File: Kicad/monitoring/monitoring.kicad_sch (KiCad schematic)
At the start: 22 parts, among them J1 Module1, J2 Module2, J3 Module3, J4 buttons, J5 Display, J6 Display, J7 DC_in_outout, U1 4052, U3 L7805, U4 L7805

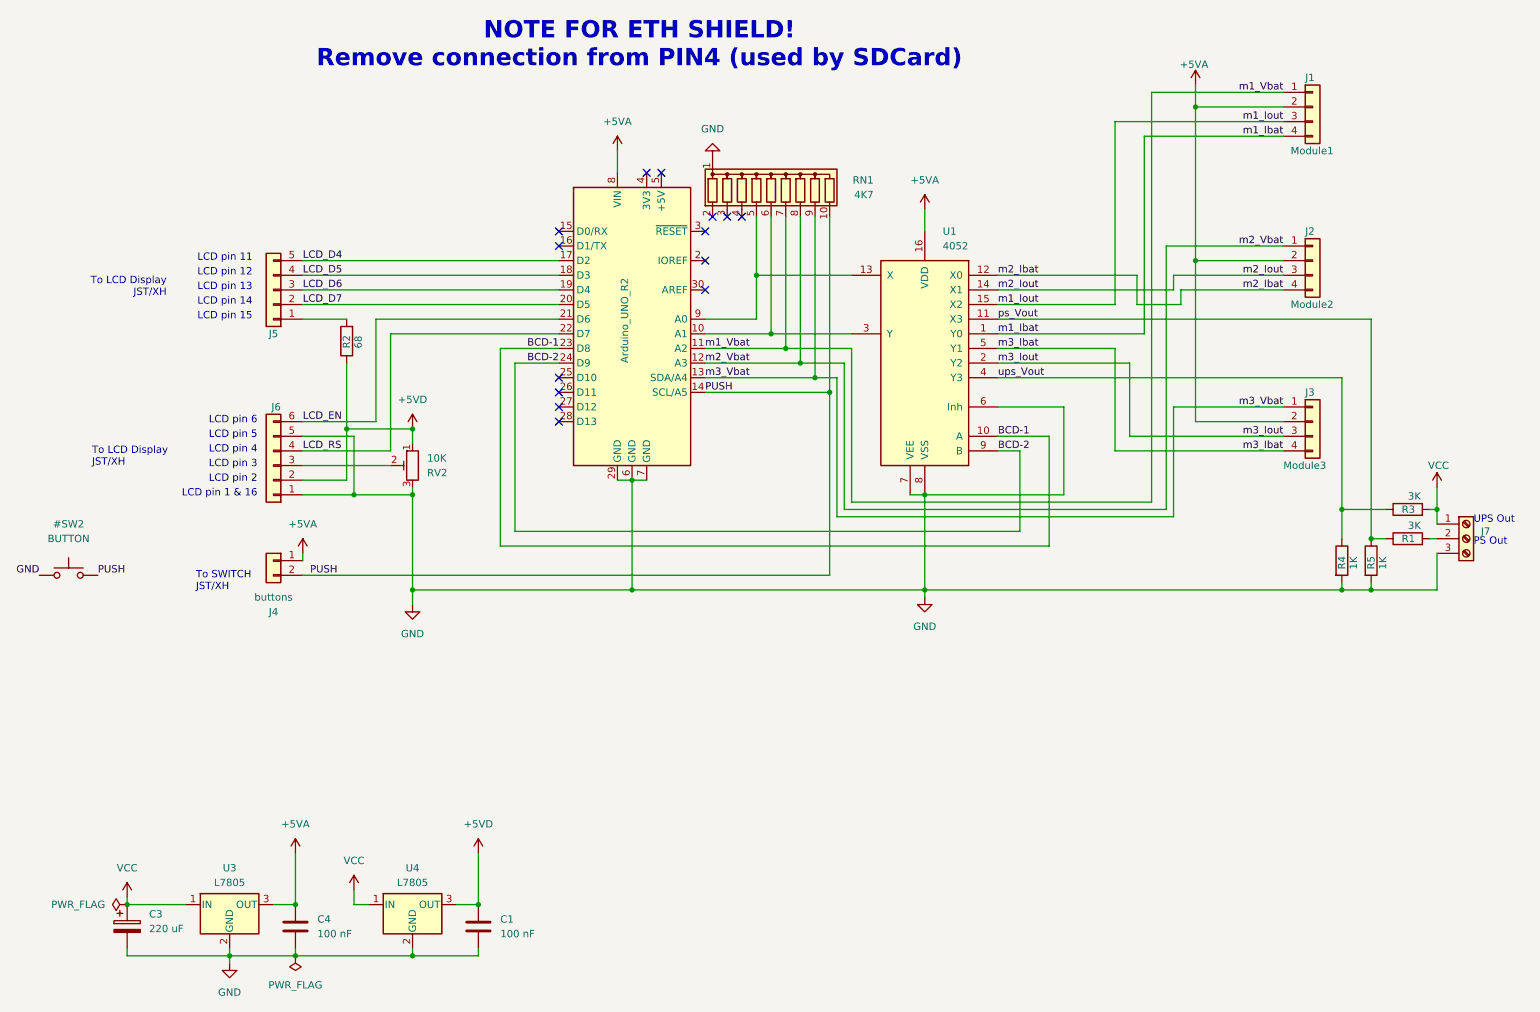
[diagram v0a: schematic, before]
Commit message: Update .sproject, io.cpp, io.h, and 29 more files
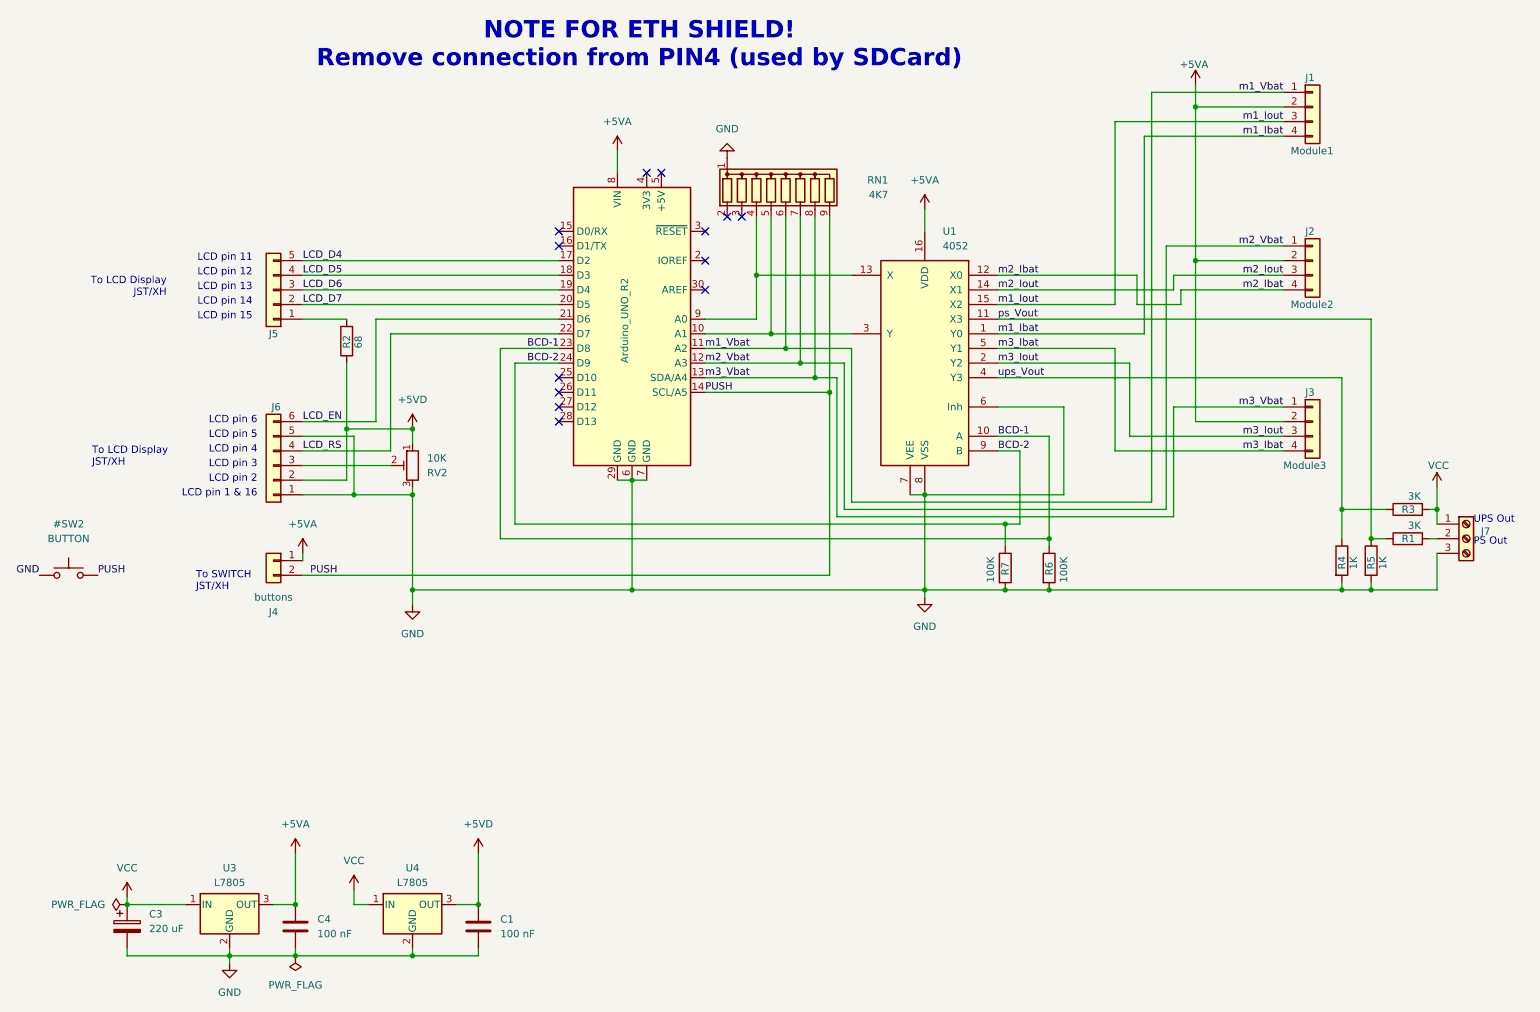
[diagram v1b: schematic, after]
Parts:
- added R6, R7: 100K, Resistor_THT:R_Axial_DIN0204_L3.6mm_D1.6mm_P7.62mm_Horizontal, symbol Device:R
- RN1: footprint Resistor_THT:R_Array_SIP10 -> Resistor_THT:R_Array_SIP8; symbol Device:R_Network09 -> Device:R_Network08
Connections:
- net BCD-1: now also R6.1
- net BCD-2: now also R7.1
- net GND: now also R6.2, R7.2
- net PUSH: now also RN1.9 (R8); no longer RN1.10 (R9)
- net m1_Vbat: now also RN1.6 (R5); no longer RN1.7 (R6)
- net m2_Vbat: now also RN1.7 (R6); no longer RN1.8 (R7)
- net m3_Vbat: now also RN1.8 (R7); no longer RN1.9 (R8)
- net at A1.10 (A1), U1.3 (Y): now also RN1.5 (R4); no longer RN1.6 (R5)
- net at A1.9 (A0), U1.13 (X): now also RN1.4 (R3); no longer RN1.5 (R4)
- no-connect marks 14 -> 13
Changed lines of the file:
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@@
 	)
 	(junction
+		(at 195.58 116.84)
+		(diameter 0)
+		(color 0 0 0 0)
+	)
+	(junction
 		(at 43.18 171.45)
 		(diameter 0)
@@
 	)
 	(junction
+		(at 203.2 116.84)
+		(diameter 0)
+		(color 0 0 0 0)
+	)
+	(junction
+		(at 195.58 105.41)
+		(diameter 0)
+		(color 0 0 0 0)
+	)
+	(junction
 		(at 60.96 180.34)
 		(diameter 0)
@@
 	)
 	(junction
+		(at 203.2 107.95)
+		(diameter 0)
+		(color 0 0 0 0)
+	)
+	(junction
 		(at 130.81 116.84)
 		(diameter 0)
@@
 	)
 	(no_connect
-		(at 144.78 52.07)
-	)
-	(no_connect
 		(at 118.11 87.63)
 	)
@@
 	(wire
 		(pts
-			(xy 110.49 106.68) (xy 198.12 106.68)
-		)
-		(stroke
-			(width 0)
-			(type default)
-		)
-	)
-	(wire
-		(pts
 			(xy 166.37 104.14) (xy 224.79 104.14)
 		)
@@
 	(wire
 		(pts
-			(xy 198.12 92.71) (xy 198.12 106.68)
+			(xy 198.12 92.71) (xy 198.12 105.41)
 		)
 		(stroke
@@
 	(wire
 		(pts
+			(xy 195.58 116.84) (xy 203.2 116.84)
+		)
+		(stroke
+			(width 0)
+			(type default)
+		)
+	)
+	(wire
+		(pts
 			(xy 269.24 107.95) (xy 270.51 107.95)
 		)
@@
 	(wire
 		(pts
+			(xy 195.58 105.41) (xy 198.12 105.41)
+		)
+		(stroke
+			(width 0)
+			(type default)
+		)
+	)
+	(wire
+		(pts
 			(xy 43.18 170.18) (xy 43.18 171.45)
 		)
@@
 	(wire
 		(pts
-			(xy 203.2 109.22) (xy 203.2 90.17)
+			(xy 203.2 109.22) (xy 203.2 107.95)
 		)
 		(stroke
@@
 	(wire
 		(pts
+			(xy 203.2 107.95) (xy 203.2 90.17)
+		)
+		(stroke
+			(width 0)
+			(type default)
+		)
+	)
+	(wire
+		(pts
 			(xy 194.31 92.71) (xy 198.12 92.71)
 		)
@@
 	(wire
 		(pts
+			(xy 110.49 105.41) (xy 195.58 105.41)
+		)
+		(stroke
+			(width 0)
+			(type default)
+		)
+	)
+	(wire
+		(pts
 			(xy 167.64 102.87) (xy 223.52 102.87)
 		)
@@
 	(wire
 		(pts
-			(xy 107.95 109.22) (xy 203.2 109.22)
-		)
-		(stroke
-			(width 0)
-			(type default)
-		)
-	)
-	(wire
-		(pts
 			(xy 220.98 30.48) (xy 243.84 30.48)
 		)
@@
 	(wire
 		(pts
-			(xy 181.61 116.84) (xy 254 116.84)
+			(xy 181.61 116.84) (xy 195.58 116.84)
 		)
 		(stroke
@@
 	(wire
 		(pts
+			(xy 203.2 116.84) (xy 254 116.84)
+		)
+		(stroke
+			(width 0)
+			(type default)
+		)
+	)
+	(wire
+		(pts
 			(xy 226.06 64.77) (xy 243.84 64.77)
 		)
@@
 	(wire
 		(pts
-			(xy 110.49 106.68) (xy 110.49 77.47)
+			(xy 194.31 69.85) (xy 259.08 69.85)
 		)
 		(stroke
@@
 	(wire
 		(pts
-			(xy 194.31 69.85) (xy 259.08 69.85)
+			(xy 214.63 92.71) (xy 243.84 92.71)
 		)
 		(stroke
@@
 	(wire
 		(pts
-			(xy 214.63 92.71) (xy 243.84 92.71)
+			(xy 270.51 102.87) (xy 270.51 105.41)
 		)
 		(stroke
@@
 	(wire
 		(pts
-			(xy 270.51 102.87) (xy 270.51 105.41)
+			(xy 130.81 97.79) (xy 130.81 116.84)
 		)
 		(stroke
@@
 	(wire
 		(pts
-			(xy 130.81 97.79) (xy 130.81 116.84)
+			(xy 72.39 162.56) (xy 72.39 171.45)
 		)
 		(stroke
@@
 	(wire
 		(pts
-			(xy 72.39 162.56) (xy 72.39 171.45)
+			(xy 168.91 101.6) (xy 220.98 101.6)
 		)
 		(stroke
@@
 	(wire
 		(pts
-			(xy 168.91 101.6) (xy 220.98 101.6)
+			(xy 152.4 52.07) (xy 152.4 62.23)
 		)
 		(stroke
@@
 	(wire
 		(pts
-			(xy 152.4 52.07) (xy 152.4 62.23)
+			(xy 195.58 105.41) (xy 195.58 109.22)
 		)
 		(stroke
@@
 	(wire
 		(pts
+			(xy 107.95 107.95) (xy 203.2 107.95)
+		)
+		(stroke
+			(width 0)
+			(type default)
+		)
+	)
+	(wire
+		(pts
+			(xy 110.49 105.41) (xy 110.49 77.47)
+		)
+		(stroke
+			(width 0)
+			(type default)
+		)
+	)
+	(wire
+		(pts
 			(xy 118.11 74.93) (xy 107.95 74.93)
 		)
@@
 	(wire
 		(pts
-			(xy 107.95 74.93) (xy 107.95 109.22)
+			(xy 107.95 74.93) (xy 107.95 107.95)
 		)
 		(stroke
@@
 	)
 	(symbol
+		(lib_id "Device:R")
+		(at 195.58 113.03 0)
+		(unit 1)
+		(exclude_from_sim no)
+		(in_bom yes)
+		(on_board yes)
+		(dnp no)
+		(property "Reference" "R7"
+			(at 195.58 114.3 90)
+			(effects
+				(font
+					(size 1.27 1.27)
+				)
+				(justify left)
+			)
+		)
+		(property "Value" "100K"
+			(at 193.04 115.57 90)
+			(effects
+				(font
+					(size 1.27 1.27)
+				)
+				(justify left)
+			)
+		)
+		(property "Footprint" "Resistor_THT:R_Axial_DIN0204_L3.6mm_D1.6mm_P7.62mm_Horizontal"
+			(at 193.802 113.03 90)
+			(effects
+				(font
+					(size 1.27 1.27)
+				)
+				(hide yes)
+			)
+		)
+		(property "Datasheet" "~"
+			(at 195.58 113.03 0)
+			(effects
+				(font
+					(size 1.27 1.27)
+				)
+				(hide yes)
+			)
+		)
+		(property "Description" "Resistor"
+			(at 195.58 113.03 0)
+			(effects
+				(font
+					(size 1.27 1.27)
+				)
+				(hide yes)
+			)
+		)
+		(pin "2"
+		)
+		(pin "1"
+		)
+		(instances
+			(project "monitoring"
+				(path "/3131f2da-09b7-4506-8682-a60f068b99cd"
+					(reference "R7")
+					(unit 1)
+				)
+			)
+		)
+	)
+	(symbol
 		(lib_id "power:PWR_FLAG")
 		(at 72.39 180.34 180)
@@
 	(symbol
 		(lib_id "power:GND")
-		(at 144.78 41.91 180)
+		(at 147.32 41.91 180)
 		(unit 1)
 		(exclude_from_sim no)
@@
 		(fields_autoplaced yes)
 		(property "Reference" "#PWR09"
-			(at 144.78 35.56 0)
+			(at 147.32 35.56 0)
 			(effects
 				(font
@@
 		)
 		(property "Value" "GND"
-			(at 144.78 36.83 0)
+			(at 147.32 36.83 0)
 			(effects
 				(font
@@
 		)
 		(property "Footprint" ""
-			(at 144.78 41.91 0)
+			(at 147.32 41.91 0)
 			(effects
 				(font
@@
 		)
 		(property "Datasheet" ""
-			(at 144.78 41.91 0)
+			(at 147.32 41.91 0)
 			(effects
 				(font
@@
 		)
 		(property "Description" "Power symbol creates a global label with name \"GND\" , ground"
-			(at 144.78 41.91 0)
+			(at 147.32 41.91 0)
 			(effects
 				(font
@@
 	)
 	(symbol
-		(lib_id "Device:R_Network09")
-		(at 154.94 46.99 0)
+		(lib_id "Device:R")
+		(at 203.2 113.03 0)
+		(unit 1)
+		(exclude_from_sim no)
+		(in_bom yes)
+		(on_board yes)
+		(dnp no)
+		(property "Reference" "R6"
+			(at 203.2 114.3 90)
+			(effects
+				(font
+					(size 1.27 1.27)
+				)
+				(justify left)
+			)
+		)
+		(property "Value" "100K"
+			(at 205.74 115.57 90)
+			(effects
+				(font
+					(size 1.27 1.27)
+				)
+				(justify left)
+			)
+		)
+		(property "Footprint" "Resistor_THT:R_Axial_DIN0204_L3.6mm_D1.6mm_P7.62mm_Horizontal"
+			(at 201.422 113.03 90)
+			(effects
+				(font
+					(size 1.27 1.27)
+				)
+				(hide yes)
+			)
+		)
+		(property "Datasheet" "~"
+			(at 203.2 113.03 0)
+			(effects
+				(font
+					(size 1.27 1.27)
+				)
+				(hide yes)
+			)
+		)
+		(property "Description" "Resistor"
+			(at 203.2 113.03 0)
+			(effects
+				(font
+					(size 1.27 1.27)
+				)
+				(hide yes)
+			)
+		)
+		(pin "2"
+		)
+		(pin "1"
+		)
+		(instances
+			(project ""
+				(path "/3131f2da-09b7-4506-8682-a60f068b99cd"
+					(reference "R6")
+					(unit 1)
+				)
+			)
+		)
+	)
+	(symbol
+		(lib_id "Device:R_Network08")
+		(at 157.48 46.99 0)
 		(unit 1)
 		(exclude_from_sim no)
@@
 		(dnp no)
 		(property "Reference" "RN1"
-			(at 172.72 45.72 0)
+			(at 175.26 45.72 0)
 			(effects
 				(font
@@
 		)
 		(property "Value" "4K7"
-			(at 172.72 48.26 0)
+			(at 175.26 48.26 0)
 			(effects
 				(font
@@
 			)
 		)
-		(property "Footprint" "Resistor_THT:R_Array_SIP10"
+		(property "Footprint" "Resistor_THT:R_Array_SIP8"
 			(at 169.545 46.99 90)
 			(effects
@@
 		)
 		(property "Datasheet" "http://www.vishay.com/docs/31509/csc.pdf"
-			(at 154.94 46.99 0)
+			(at 157.48 46.99 0)
 			(effects
 				(font
@@
 			)
 		)
-		(property "Description" "9 resistor network, star topology, bussed resistors, small symbol"
-			(at 154.94 46.99 0)
+		(property "Description" "8 resistor network, star topology, bussed resistors, small symbol"
+			(at 157.48 46.99 0)
 			(effects
 				(font
@@
 		(pin "9"
 		)
-		(pin "10"
-		)
 		(pin "6"
